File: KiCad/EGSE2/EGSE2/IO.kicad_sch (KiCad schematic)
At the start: 4 parts, among them J1 USB_C_Receptacle_USB2.0_16P, J2 USB_C_Receptacle_USB2.0_16P, J3 DA15_Socket_MountingHoles, J4 Conn_02x08_Top_Bottom

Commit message: gamig on this EGSE type hsi
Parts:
- J1, J2: footprint Connector_USB:USB_C_Receptacle_GCT_USB4105-xx-A_16P_TopMnt_Horizontal -> Connector_USB:USB_C_Receptacle_GCT_USB4085
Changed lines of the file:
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@@
 			)
 		)
-		(property "Footprint" "Connector_USB:USB_C_Receptacle_GCT_USB4105-xx-A_16P_TopMnt_Horizontal"
+		(property "Footprint" "Connector_USB:USB_C_Receptacle_GCT_USB4085"
 			(at 52.07 55.88 0)
 			(effects
@@
 			)
 		)
-		(property "Footprint" "Connector_USB:USB_C_Receptacle_GCT_USB4105-xx-A_16P_TopMnt_Horizontal"
+		(property "Footprint" "Connector_USB:USB_C_Receptacle_GCT_USB4085"
 			(at 52.07 114.3 0)
 			(effects

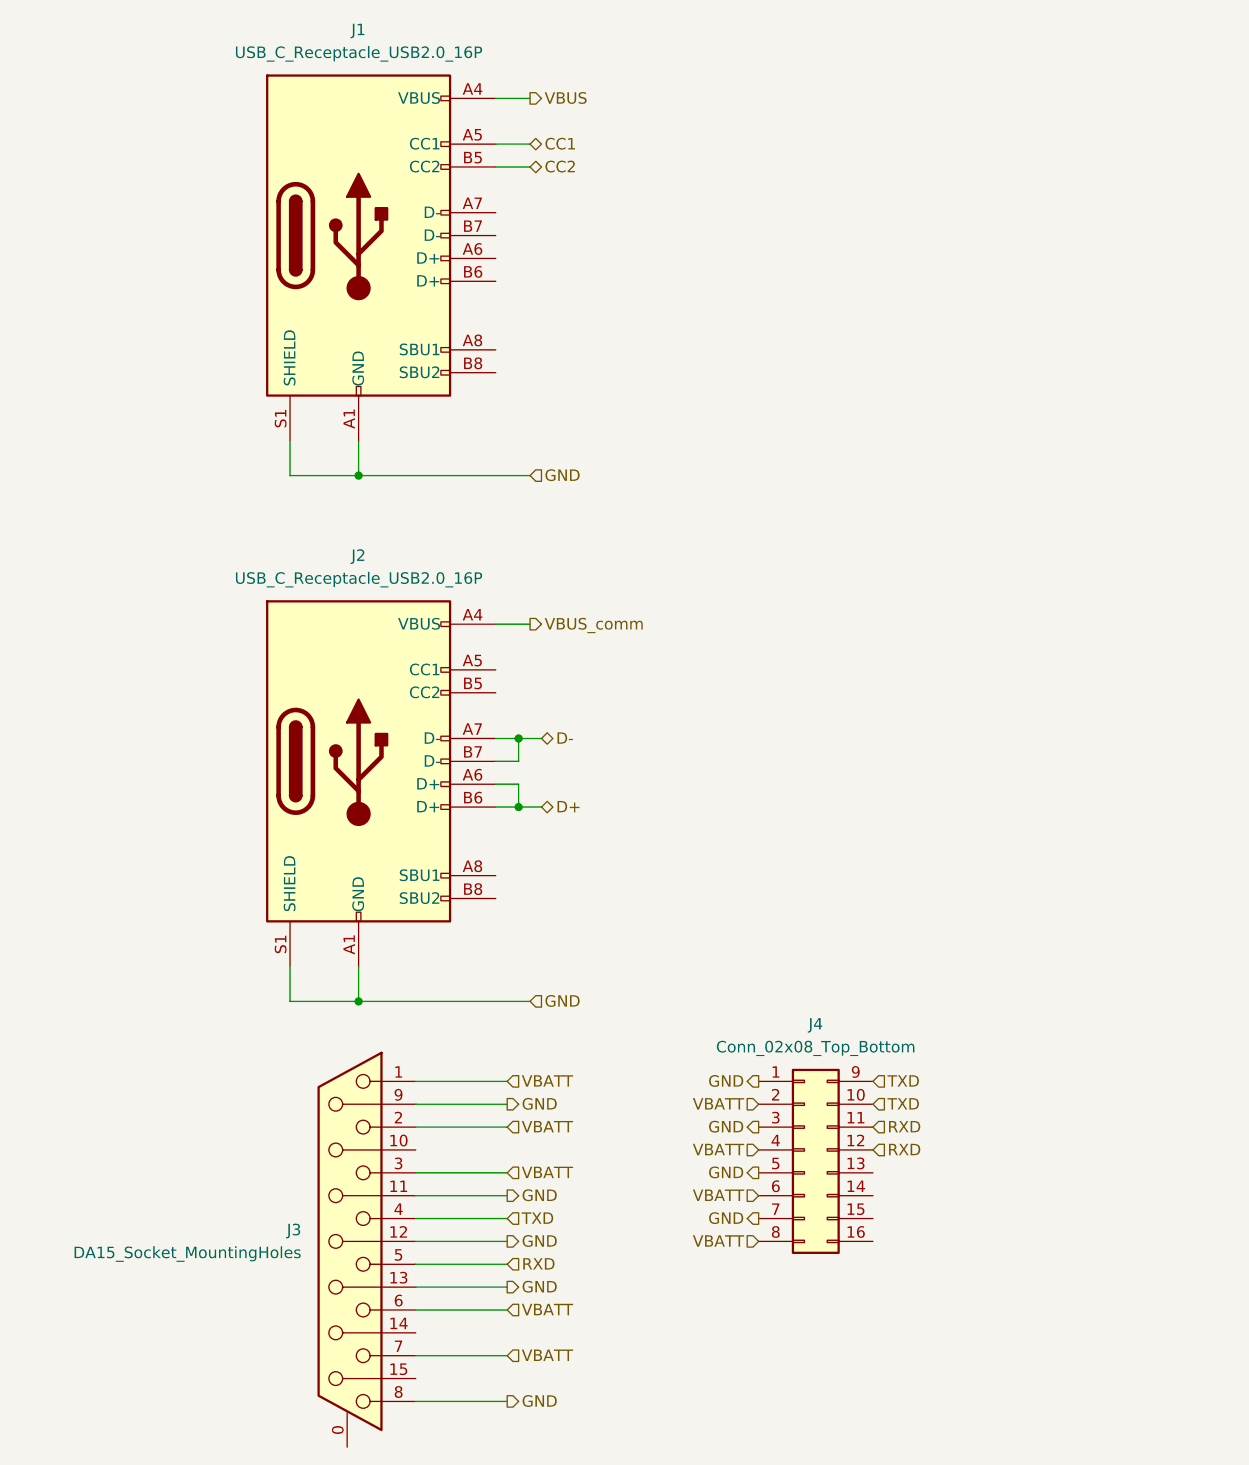
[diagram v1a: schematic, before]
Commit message: ewo
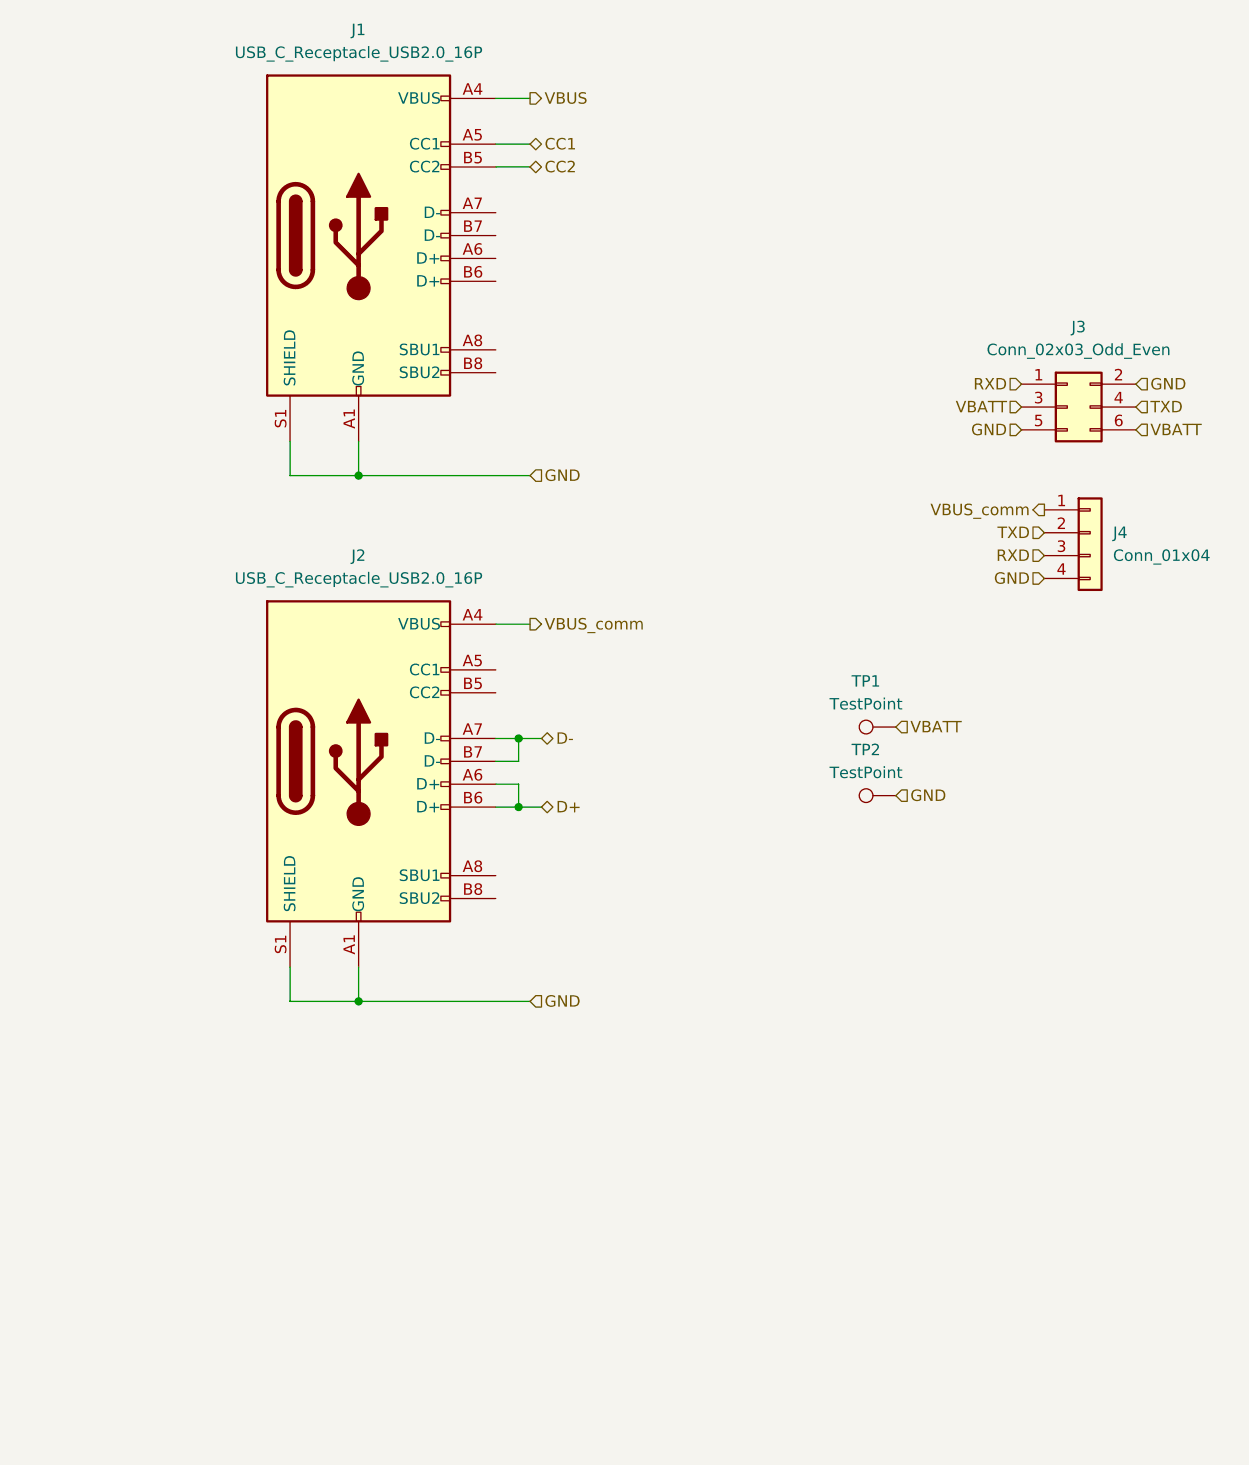
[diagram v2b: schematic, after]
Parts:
- removed J3: DA15_Socket_MountingHoles, Connector_Dsub:DSUB-15-HD_Socket_Horizontal_P2.29x2.54mm_EdgePinOffset8.35mm_Housed_MountingHolesOffset10.89mm, symbol Connector:DA15_Socket_MountingHoles
- removed J4: Conn_02x08_Top_Bottom, Connector_PinHeader_2.54mm:PinHeader_2x08_P2.54mm_Vertical, symbol Connector_Generic:Conn_02x08_Top_Bottom
- added J3: Conn_02x03_Odd_Even, C6:CONN_SD-44764-001_06_MOL, symbol Connector_Generic:Conn_02x03_Odd_Even
- added J4: Conn_01x04, Connector:FanPinHeader_1x04_P2.54mm_Vertical, symbol Connector_Generic:Conn_01x04
- added TP1, TP2: TestPoint, TestPoint:TestPoint_Keystone_5019_Miniature, symbol Connector:TestPoint
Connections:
- net GND: now also J3.2 (Pin_2), J3.5 (Pin_5), J4.4 (Pin_4), TP2.1
- net RXD: now also J3.1 (Pin_1), J4.3 (Pin_3)
- net TXD: now also J3.4 (Pin_4), J4.2 (Pin_2)
- net VBATT: now also J3.3 (Pin_3), J3.6 (Pin_6), TP1.1
- net VBUS_comm: now also J4.1 (Pin_1)
